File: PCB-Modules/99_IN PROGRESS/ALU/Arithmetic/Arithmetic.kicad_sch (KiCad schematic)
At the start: 26 parts, among them J1 Conn_01x08, J2 Conn_01x08, J3 Conn_01x08, J4 Conn_01x08, U1 74LS157, U2 74LS157, U3 74LS86, U32 74LS04, U33 74LS08, U34 74LS32, U4 74LS86, U5 74LS283, U6 74LS283, U7 74LS245

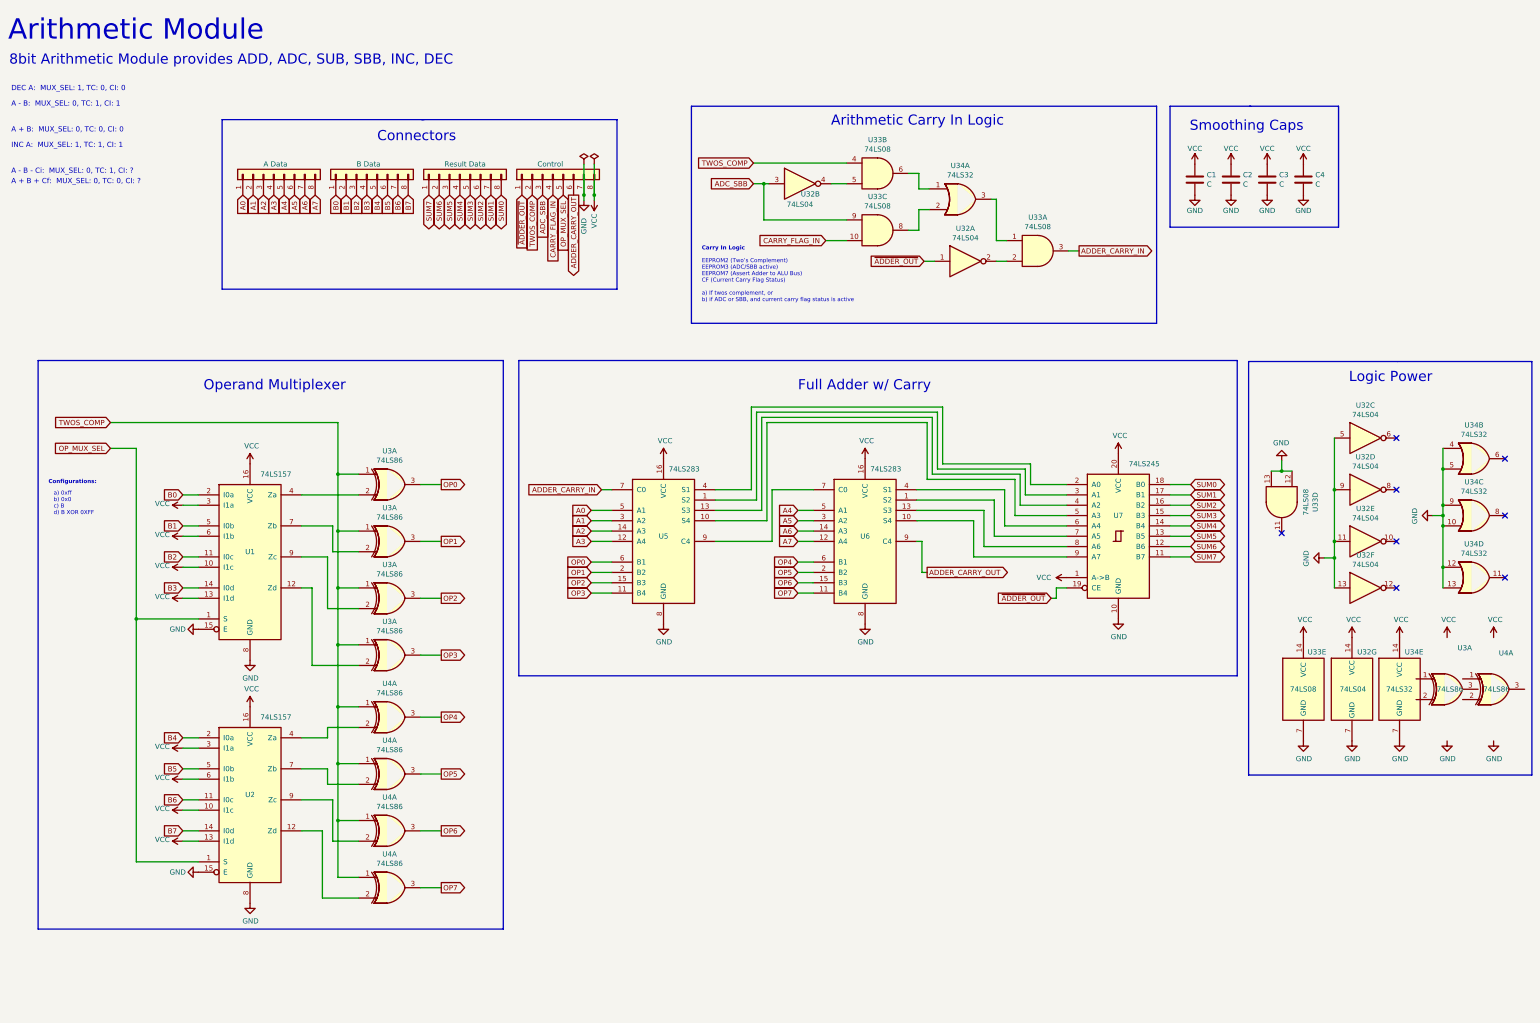
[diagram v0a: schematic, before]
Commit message: Documentation and Cleanup
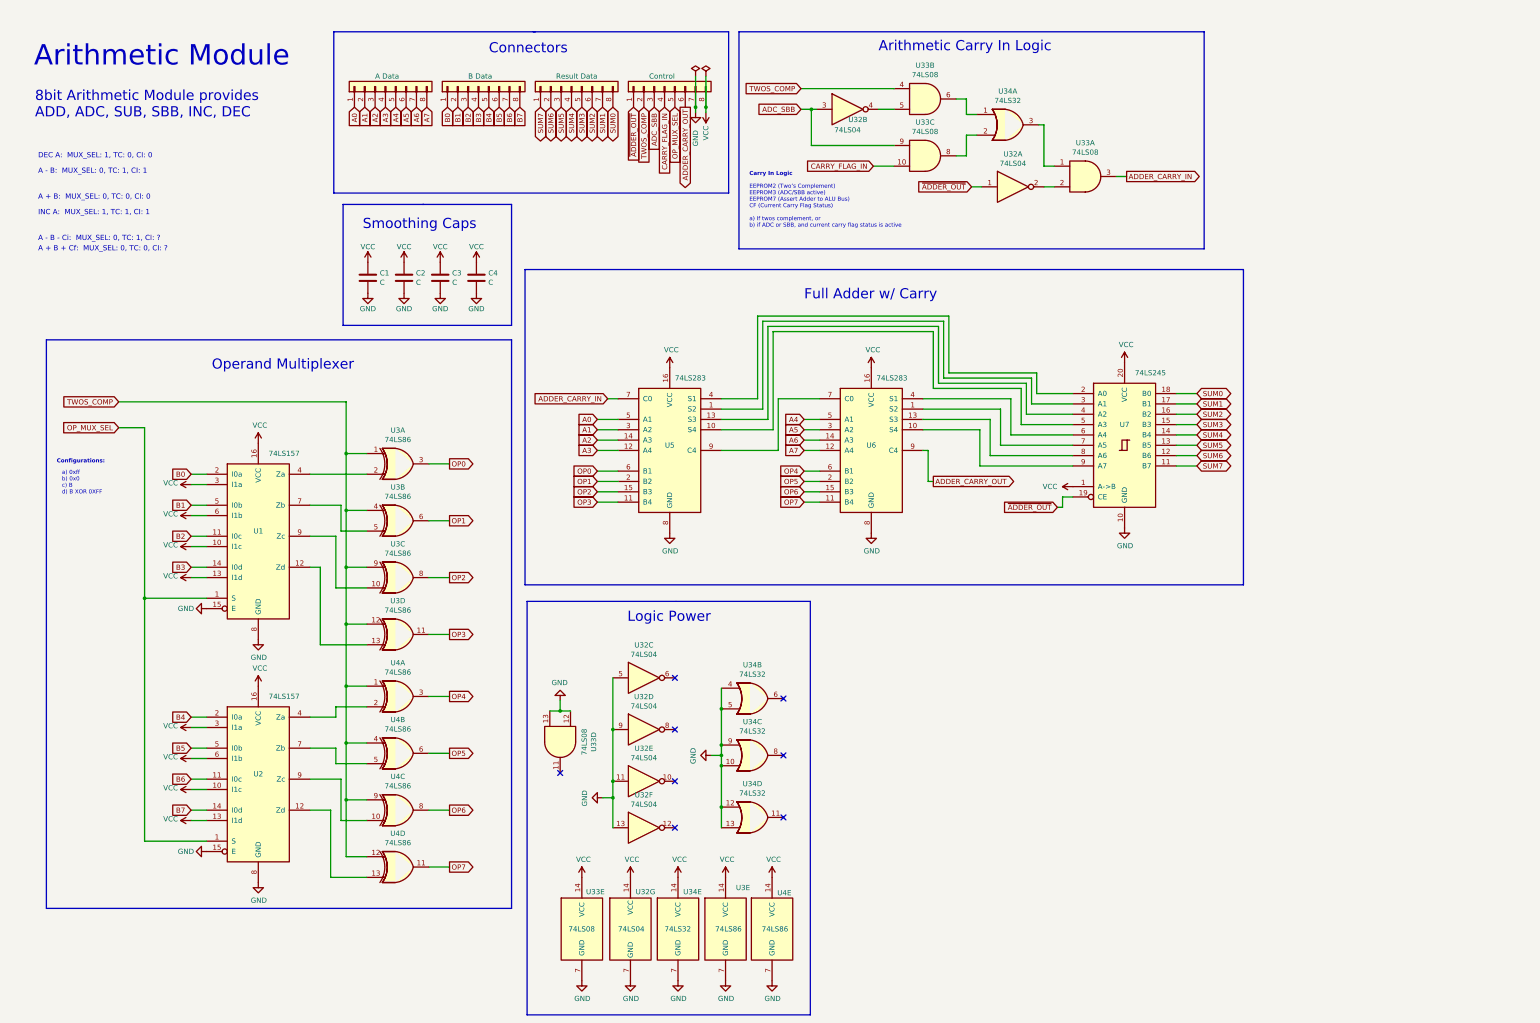
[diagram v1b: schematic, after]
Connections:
- net GND: now also U3.7 (GND), U4.7 (GND)
- net OP1: now also U3.6; no longer U3.3
- net OP2: now also U3.8; no longer U3.3
- net OP3: now also U3.11; no longer U3.3
- net OP5: now also U4.6; no longer U4.3
- net OP6: now also U4.8; no longer U4.3
- net OP7: now also U4.11; no longer U4.3
- net TWOS_COMP: now also U3.12, U3.4, U3.9, U4.12, U4.4, U4.9; no longer U3.1, U3.1, U3.1, U4.1, U4.1, U4.1
- net VCC: now also U3.14 (VCC), U4.14 (VCC)
- net at U2.12 (Zd): now also U4.13; no longer U4.2
- net at U2.7 (Zb): now also U4.5; no longer U4.2
- net at U2.9 (Zc): now also U4.10; no longer U4.2
- net at U1.12 (Zd): now also U3.13; no longer U3.2
- net at U1.7 (Zb): now also U3.5; no longer U3.2
- net at U1.9 (Zc): now also U3.10; no longer U3.2
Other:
- moved on the sheet: C1, C2, C3, C4, U1, U2, U32A, U32B, U32C, U32D, U32E, U32F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
